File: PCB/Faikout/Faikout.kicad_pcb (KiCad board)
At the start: 2 copper layers, 70 x 70 mm, 44 parts, among them J1 S21, J2 TC2030-USB-NL, J3 Reset, Q1 BSS138PS, U1 TPS62933, U4 ESP32-S3-MINI-1

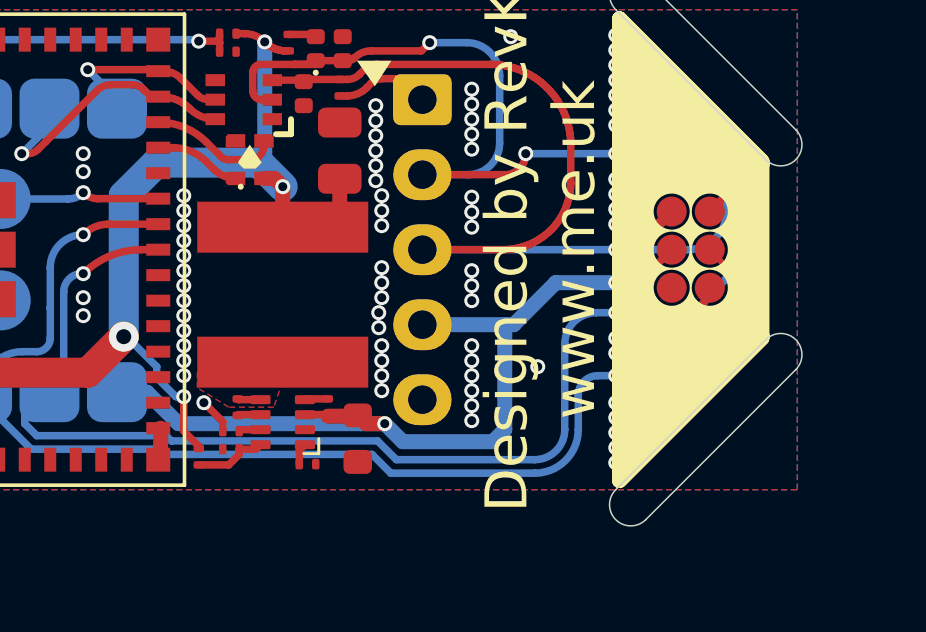
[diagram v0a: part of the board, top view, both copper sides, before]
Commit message: Tweaks
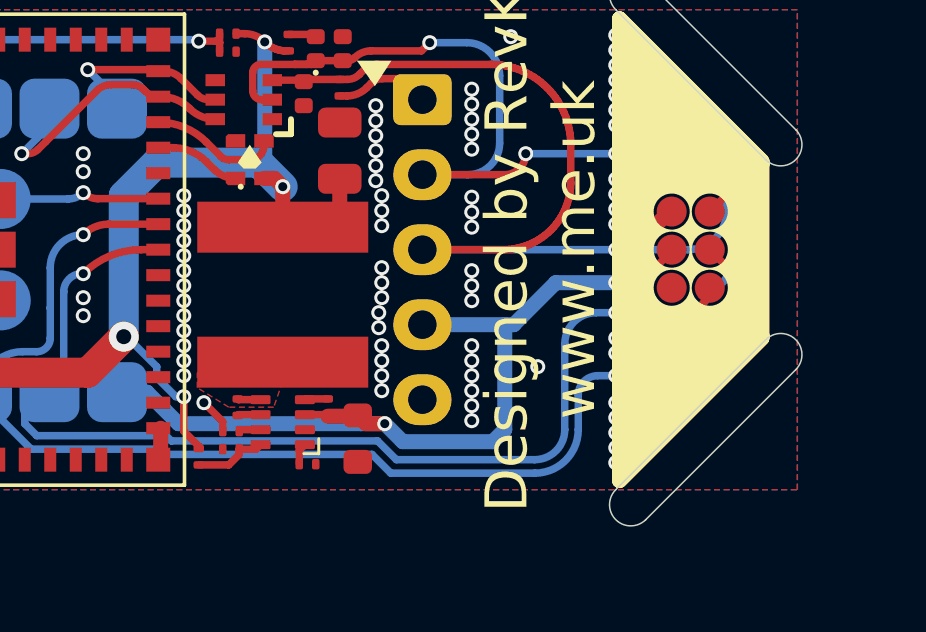
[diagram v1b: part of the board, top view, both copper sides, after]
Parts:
- turned FID3 to 180 degrees
